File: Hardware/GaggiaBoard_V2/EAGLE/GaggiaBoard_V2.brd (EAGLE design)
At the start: 102 x 92 mm, 115 parts, among them IC1 LD117AS33TR, IC2 LD117AS33TR, J11 PIN262409-1, J12 PIN262409-1, J13 PIN262409-1, J14 PIN262409-1, J15 PIN262409-1, J16 PIN262409-1, J17 PIN262409-1, J18 PIN262409-1, J19 PIN262409-1, J2 Vertical Qwiic Connector, J20 PIN262409-1, J24 5033981892, J3 Vertical Qwiic Connector, J5 2PIN, J6 3PIN, J7 3PIN, J8 5PIN, J9 3PIN, K1 RELAY-SPDT-JZC-11F, K2 RELAY-SPDT-JZC-11F, K3 RELAY-SPDT-JZC-11F, Q1 600mA/40V, Q10 600mA/40V, Q2 600mA/40V, Q3 600mA/40V, Q4 600mA/40V, Q5 600mA/40V, Q6 600mA/40V, Q8 600mA/40V, Q9 600mA/40V, U1 BLACKPILL, U2 MAX31855K, U5 TXS0102

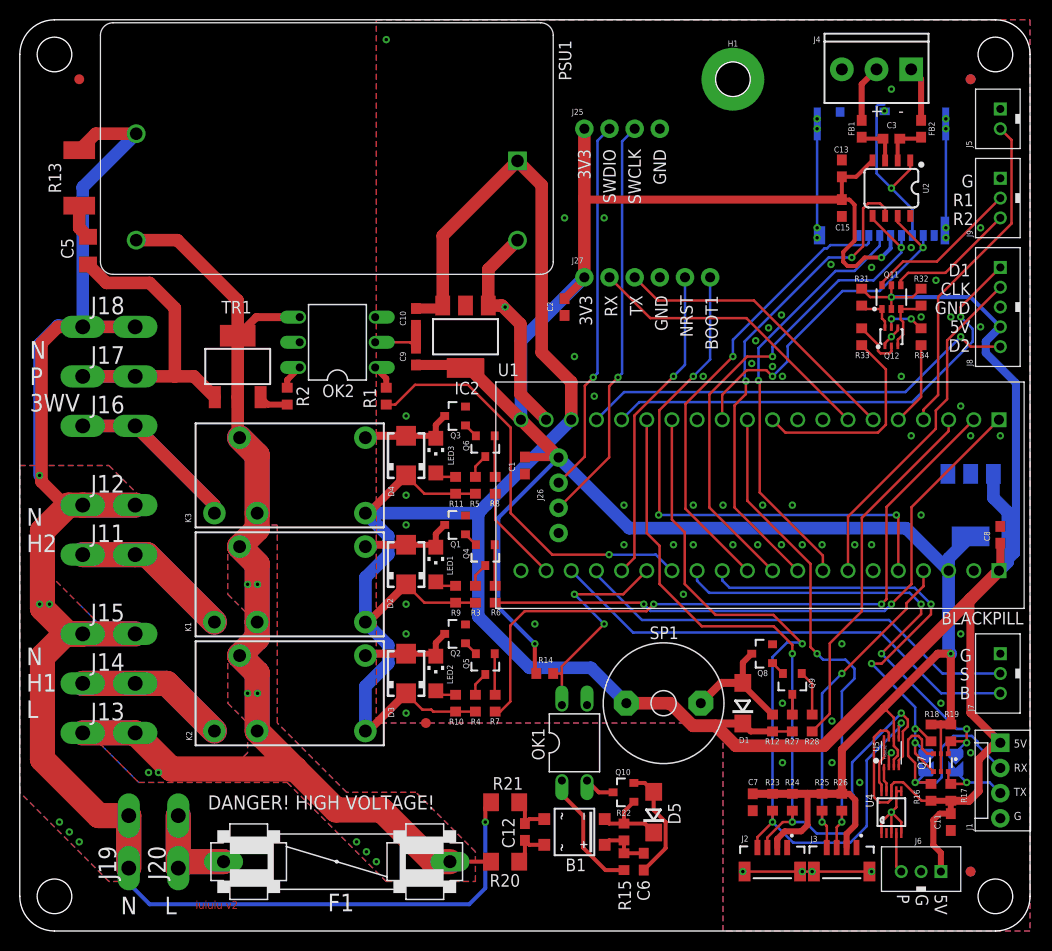
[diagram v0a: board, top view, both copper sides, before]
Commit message: part list fix
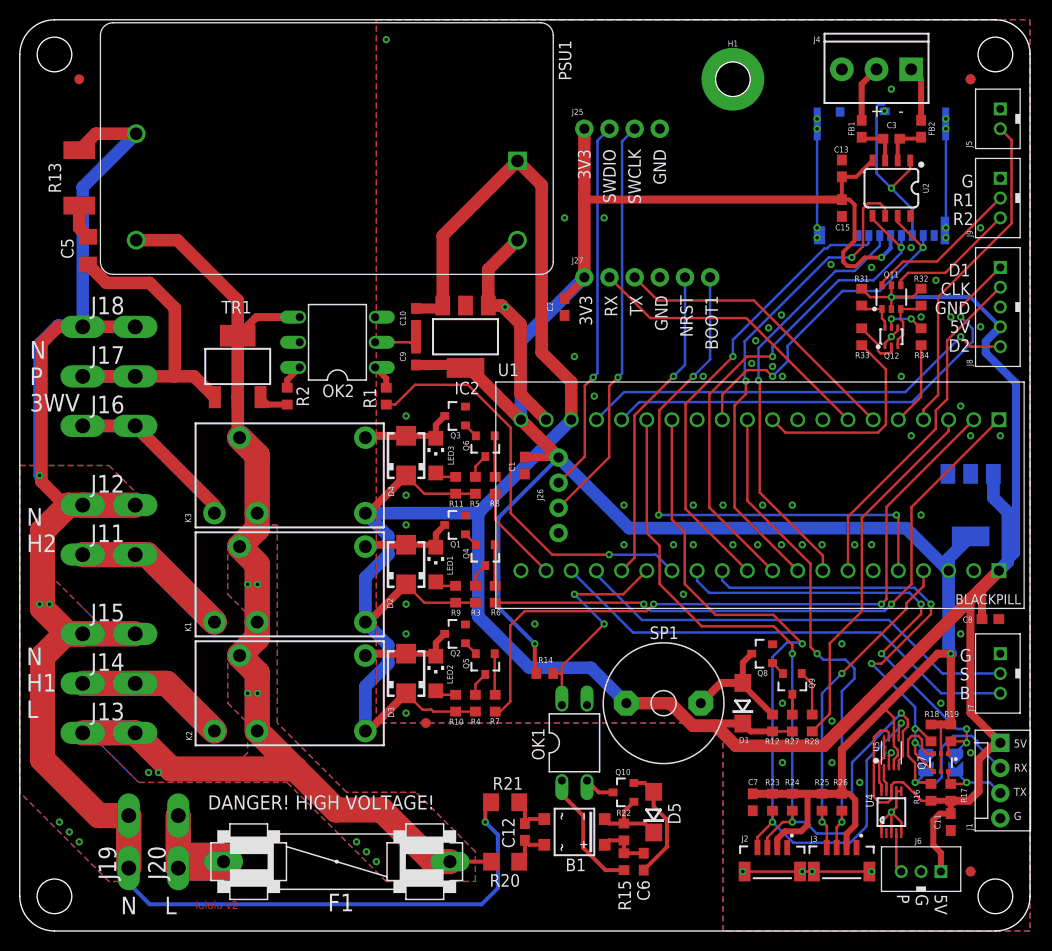
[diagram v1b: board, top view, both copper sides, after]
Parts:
- moved C8 8.56 mm to (92.0, 25.5), turned to 0 degrees
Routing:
- net 5V: track 344.2 -> 347.0 mm
- net AC_N: track 205.5 -> 207.3 mm
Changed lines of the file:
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@@
 <drawing>
 <settings>
-<setting alwaysvectorfont="yes"/>
+<setting alwaysvectorfont="no"/>
 <setting verticaltext="up"/>
 </settings>
@@
 </layers>
 <board>
-<fusionsync huburn="a.YnVzaW5lc3M6Z21haWwyMjIzNTY5" projecturn="a.YnVzaW5lc3M6Z21haWwyMjIzNTY5I0QyMDIyMDEwNDQ4MTQ5MTcwNg" f3durn="urn:adsk.wipprod:dm.lineage:6w6Byw4bTdmTaueqAgbUEw" pcbguid="" lastpulledtime="" lastsyncedchangeguid="" latestrevisionid="172b21af-06b0-469f-97ae-7bcfc94109dc" lastsyncedrevisionid="172b21af-06b0-469f-97ae-7bcfc94109dc" lastboardhashguid="f24e53fc-158b-1f6d-4315-241966646160" lastpushedtime="2022-07-08T06:02:15Z" linktopcb3d="true"/>
+<fusionsync huburn="a.YnVzaW5lc3M6Z21haWwyMjIzNTY5" projecturn="a.YnVzaW5lc3M6Z21haWwyMjIzNTY5I0QyMDIyMDEwNDQ4MTQ5MTcwNg" f3durn="urn:adsk.wipprod:dm.lineage:6w6Byw4bTdmTaueqAgbUEw" pcbguid="" lastpulledtime="" lastsyncedchangeguid="" latestrevisionid="f5b72319-5f83-45ac-8c5c-21c1cc47dbd0" lastsyncedrevisionid="f5b72319-5f83-45ac-8c5c-21c1cc47dbd0" lastboardhashguid="f5f3250e-0ac0-ee41-2de5-6bbe57c72a9f" lastpushedtime="2022-08-14T00:36:34Z" linktopcb3d="true"/>
 <plain>
 <wire x1="-2.5" y1="-6" x2="92.5" y2="-6" width="0" layer="20"/>
@@
 <attribute name="VALUE" x="66.095" y="7.635" size="1.27" layer="27" rot="R270"/>
 </element>
-<element name="C8" library="rcl" library_urn="urn:adsk.eagle:library:334" package="C0603" package3d_urn="urn:adsk.eagle:package:23616/2" value="10uF/16V" x="93" y="34" smashed="yes" rot="R90">
-<attribute name="LCSC" value="C86275" x="235.24" y="116.55" size="1.778" layer="27" rot="R90" display="off"/>
-<attribute name="NAME" x="91.965" y="33.365" size="0.6096" layer="25" rot="R90"/>
-<attribute name="POPULARITY" value="37" x="235.24" y="116.55" size="1.778" layer="27" rot="R90" display="off"/>
-<attribute name="SPICEPREFIX" value="C" x="235.24" y="116.55" size="1.778" layer="27" rot="R90" display="off"/>
-<attribute name="VALUE" x="94.905" y="33.365" size="1.27" layer="27" rot="R90"/>
+<element name="C8" library="rcl" library_urn="urn:adsk.eagle:library:334" package="C0603" package3d_urn="urn:adsk.eagle:package:23616/2" value="10uF/16V" x="92" y="25.5" smashed="yes">
+<attribute name="LCSC" value="C86275" x="174.55" y="-116.74" size="1.778" layer="27" display="off"/>
+<attribute name="NAME" x="89.206" y="25.138" size="0.6096" layer="25"/>
+<attribute name="POPULARITY" value="37" x="174.55" y="-116.74" size="1.778" layer="27" display="off"/>
+<attribute name="SPICEPREFIX" value="C" x="174.55" y="-116.74" size="1.778" layer="27" display="off"/>
+<attribute name="VALUE" x="91.365" y="23.595" size="1.27" layer="27"/>
 </element>
 <element name="C9" library="rcl" library_urn="urn:adsk.eagle:library:334" package="C0603" package3d_urn="urn:adsk.eagle:package:23616/2" value="10uF/16V" x="34" y="52" smashed="yes" rot="R90">
@@
 </element>
 <element name="IC1" library="v-reg" library_urn="urn:adsk.eagle:library:409" package="SOT223" package3d_urn="urn:adsk.eagle:package:30370/1" override_package3d_urn="urn:adsk.eagle:package:36461295/2" override_package_urn="urn:adsk.eagle:footprint:30315/1" value="LD117AS33TR" x="90" y="37" smashed="yes" rot="MR180">
-<attribute name="LCSC" value="C152529" x="209.38" y="125.9" size="1.778" layer="28" rot="MR180" display="off"/>
+<attribute name="LCSC" value="C26537" x="209.38" y="125.9" size="1.778" layer="28" rot="MR180" display="off"/>
 <attribute name="NAME" x="88.66" y="43.1492" size="1.27" layer="26" rot="MR180"/>
 <attribute name="POPULARITY" value="9" x="209.38" y="125.9" size="1.778" layer="28" rot="MR180" display="off"/>
@@
 </element>
 <element name="IC2" library="v-reg" library_urn="urn:adsk.eagle:library:409" package="SOT223" package3d_urn="urn:adsk.eagle:package:30370/1" override_package3d_urn="urn:adsk.eagle:package:36461293/2" override_package_urn="urn:adsk.eagle:footprint:30315/1" value="LD117AS33TR" x="39" y="54" smashed="yes" rot="R180">
-<attribute name="LCSC" value="C152529" x="16.14" y="163.22" size="1.778" layer="27" rot="R180" display="off"/>
+<attribute name="LCSC" value="C26537" x="16.14" y="163.22" size="1.778" layer="27" rot="R180" display="off"/>
 <attribute name="NAME" x="40.44" y="49.4492" size="1.27" layer="25" rot="R180"/>
 <attribute name="POPULARITY" value="9" x="16.14" y="163.22" size="1.778" layer="27" rot="R180" display="off"/>
@@
 </element>
 <element name="LED1" library="adafruit" library_urn="urn:adsk.eagle:library:420" package="CHIPLED_1206" package3d_urn="urn:adsk.eagle:package:6240560/1" override_package3d_urn="urn:adsk.eagle:package:36462256/4" override_package_urn="urn:adsk.eagle:footprint:6239914/1" value="" x="36" y="31" smashed="yes">
-<attribute name="LCSC" value="C375534" x="163" y="-96" size="1.778" layer="27" display="off"/>
+<attribute name="LCSC" value="C125086" x="163" y="-96" size="1.778" layer="27" display="off"/>
 <attribute name="NAME" x="37.73" y="29.93" size="0.6096" layer="25" rot="R90"/>
 <attribute name="VALUE" x="38.54" y="29.73" size="1.27" layer="27" rot="R90"/>
 </element>
 <element name="LED2" library="adafruit" library_urn="urn:adsk.eagle:library:420" package="CHIPLED_1206" package3d_urn="urn:adsk.eagle:package:6240560/1" override_package3d_urn="urn:adsk.eagle:package:36462272/2" override_package_urn="urn:adsk.eagle:footprint:6239914/1" value="" x="36" y="20" smashed="yes">
-<attribute name="LCSC" value="C375534" x="49.97" y="-115.89" size="1.778" layer="27" display="off"/>
+<attribute name="LCSC" value="C125086" x="49.97" y="-115.89" size="1.778" layer="27" display="off"/>
 <attribute name="NAME" x="37.73" y="18.93" size="0.6096" layer="25" rot="R90"/>
 <attribute name="VALUE" x="38.54" y="18.73" size="1.27" layer="27" rot="R90"/>
 </element>
 <element name="LED3" library="adafruit" library_urn="urn:adsk.eagle:library:420" package="CHIPLED_1206" package3d_urn="urn:adsk.eagle:package:6240560/1" override_package3d_urn="urn:adsk.eagle:package:36462279/2" override_package_urn="urn:adsk.eagle:footprint:6239914/1" value="" x="36" y="42" smashed="yes">
-<attribute name="LCSC" value="C375534" x="55.05" y="-93.89" size="1.778" layer="27" display="off"/>
+<attribute name="LCSC" value="C125086" x="55.05" y="-93.89" size="1.778" layer="27" display="off"/>
 <attribute name="NAME" x="37.83" y="41.03" size="0.6096" layer="25" rot="R90"/>
 <attribute name="VALUE" x="38.54" y="40.73" size="1.27" layer="27" rot="R90"/>
@@
 <element name="U1" library="discrete" library_urn="urn:adsk.eagle:library:211" package="BLACKPILL" override_package3d_urn="urn:adsk.eagle:package:36462313/2" override_package_urn="urn:adsk.eagle:footprint:36462314/1" value="BLACKPILL" x="70" y="38" smashed="yes" rot="R180">
 <attribute name="NAME" x="44.4" y="51.3" size="1.27" layer="21" rot="R180"/>
-<attribute name="VALUE" x="95.342" y="26.224" size="1.27" layer="21" rot="R180"/>
+<attribute name="VALUE" x="95.088" y="28.002" size="1.016" layer="21" rot="R180"/>
 </element>
 <element name="U2" library="SparkFun-IC-Conversion" package="SO08" override_package3d_urn="urn:adsk.eagle:package:36462208/2" override_package_urn="urn:adsk.eagle:footprint:36462209/1" value="MAX31855K" x="82" y="69" smashed="yes" rot="R180">
@@
 <wire x1="92.3" y1="37.737" x2="92.3" y2="40.15" width="1.27" layer="16"/>
 <contactref element="C8" pad="1"/>
-<wire x1="93" y1="33.15" x2="93" y2="30.52" width="0.8128" layer="1"/>
-<wire x1="93" y1="30.52" x2="92.86" y2="30.38" width="0.8128" layer="1"/>
+<wire x1="92.86" y1="30.38" x2="91.15" y2="28.67" width="0.8128" layer="1"/>
+<wire x1="91.15" y1="28.67" x2="91.15" y2="25.5" width="0.8128" layer="1"/>
 </signal>
 <signal name="3V3">
@@
 <wire x1="41" y1="5" x2="41" y2="6.422" width="0.4064" layer="1"/>
 <wire x1="41" y1="6.422" x2="41.578" y2="7" width="0.4064" layer="1"/>
-<wire x1="41" y1="5" x2="41" y2="-1.672" width="0.4064" layer="16"/>
+<wire x1="41" y1="5" x2="42.27" y2="3.73" width="0.4064" layer="16"/>
+<wire x1="42.27" y1="3.73" x2="42.27" y2="-1.672" width="0.4064" layer="16"/>
 <wire x1="5" y1="-1.19" x2="5" y2="0.35" width="0.4064" layer="16"/>
-<wire x1="41" y1="-1.672" x2="39.37" y2="-3.302" width="0.4064" layer="16"/>
-<wire x1="39.37" y1="-3.302" x2="7.112" y2="-3.302" width="0.4064" layer="16"/>
+<wire x1="42.27" y1="-1.672" x2="40.64" y2="-3.302" width="0.4064" layer="16"/>
+<wire x1="40.64" y1="-3.302" x2="7.112" y2="-3.302" width="0.4064" layer="16"/>
 <wire x1="7.112" y1="-3.302" x2="5" y2="-1.19" width="0.4064" layer="16"/>
 <polygon width="0.254" layer="16">
@@
 <contactref element="D5" pad="A"/>
 <contactref element="C6" pad="2"/>
-<wire x1="58" y1="6.20289375" x2="58" y2="8.05" width="0.4064" layer="1"/>
-<wire x1="59.2056" y1="4.99729375" x2="58" y2="6.20289375" width="0.4064" layer="1"/>
-<wire x1="57" y1="0.15" x2="59.2056" y2="2.3556" width="0.4064" layer="1"/>
-<wire x1="59.2056" y1="2.3556" x2="59.2056" y2="4.99729375" width="0.4064" layer="1"/>
+<wire x1="58" y1="6.58389375" x2="58" y2="8.05" width="0.4064" layer="1"/>
+<wire x1="59.3326" y1="5.25129375" x2="58" y2="6.58389375" width="0.4064" layer="1"/>
+<wire x1="57" y1="0.15" x2="59.3326" y2="2.4826" width="0.4064" layer="1"/>
+<wire x1="59.3326" y1="2.4826" x2="59.3326" y2="5.25129375" width="0.4064" layer="1"/>
 <wire x1="56" y1="8.95" x2="57.1" y2="8.95" width="0.4064" layer="1"/>
 <wire x1="57.1" y1="8.95" x2="58" y2="8.05" width="0.4064" layer="1"/>
@@
 <wire x1="10" y1="5.65" x2="10" y2="0.35" width="2.54" layer="1"/>
 <wire x1="10" y1="0.35" x2="10.65" y2="1" width="2.54" layer="1"/>
-<wire x1="10.65" y1="1" x2="14.57" y2="1" width="2.54" layer="1"/>
+<wire x1="10.65" y1="1" x2="14.57" y2="1" width="3.81" layer="1"/>
 <wire x1="10" y1="5.65" x2="10" y2="0.35" width="2.54" layer="16"/>
 <wire x1="10" y1="0.35" x2="10.65" y2="1" width="2.54" layer="16"/>
-<wire x1="10.65" y1="1" x2="14.57" y2="1" width="2.54" layer="16"/>
+<wire x1="10.65" y1="1" x2="14.57" y2="1" width="3.81" layer="16"/>
 </signal>
 </signals>
